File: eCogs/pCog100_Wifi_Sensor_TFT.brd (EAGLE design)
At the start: 47.5 x 28 mm, 30 parts

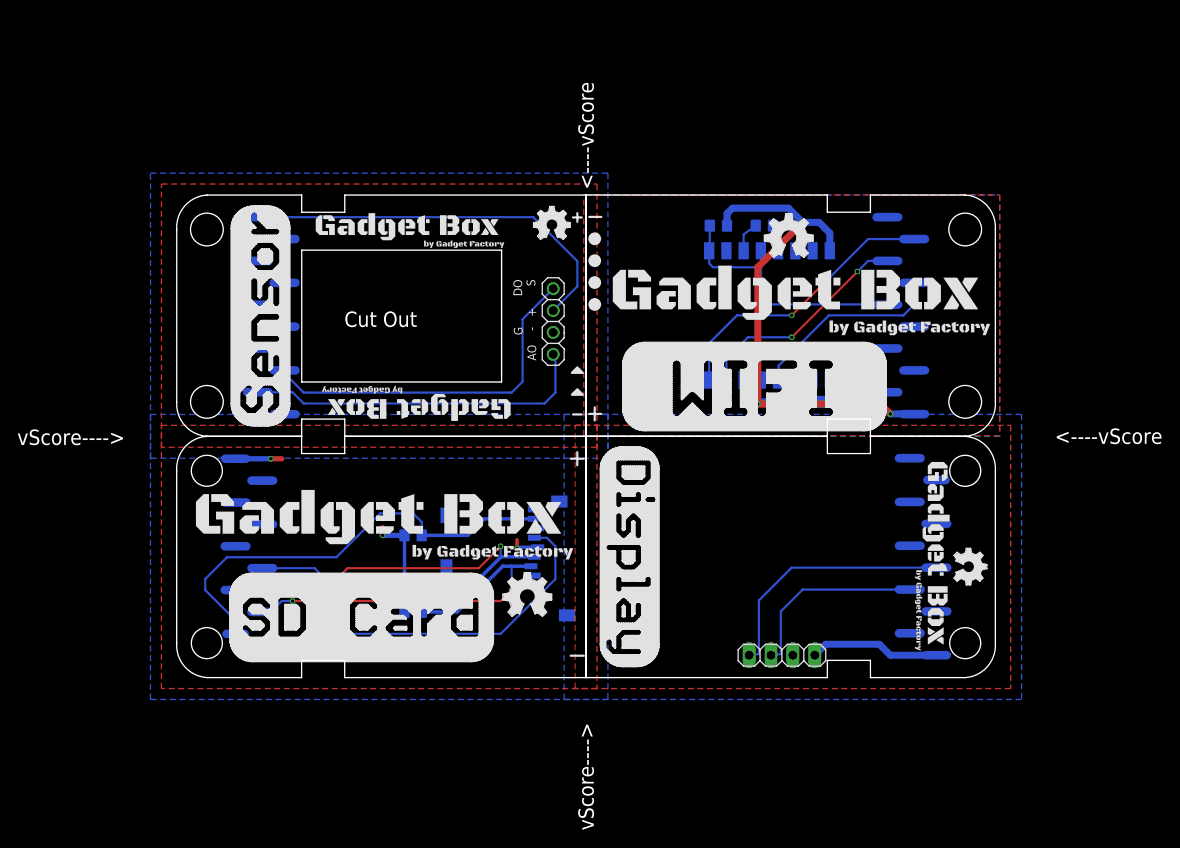
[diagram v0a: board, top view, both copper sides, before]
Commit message: pCog for Sensor Version 1.1
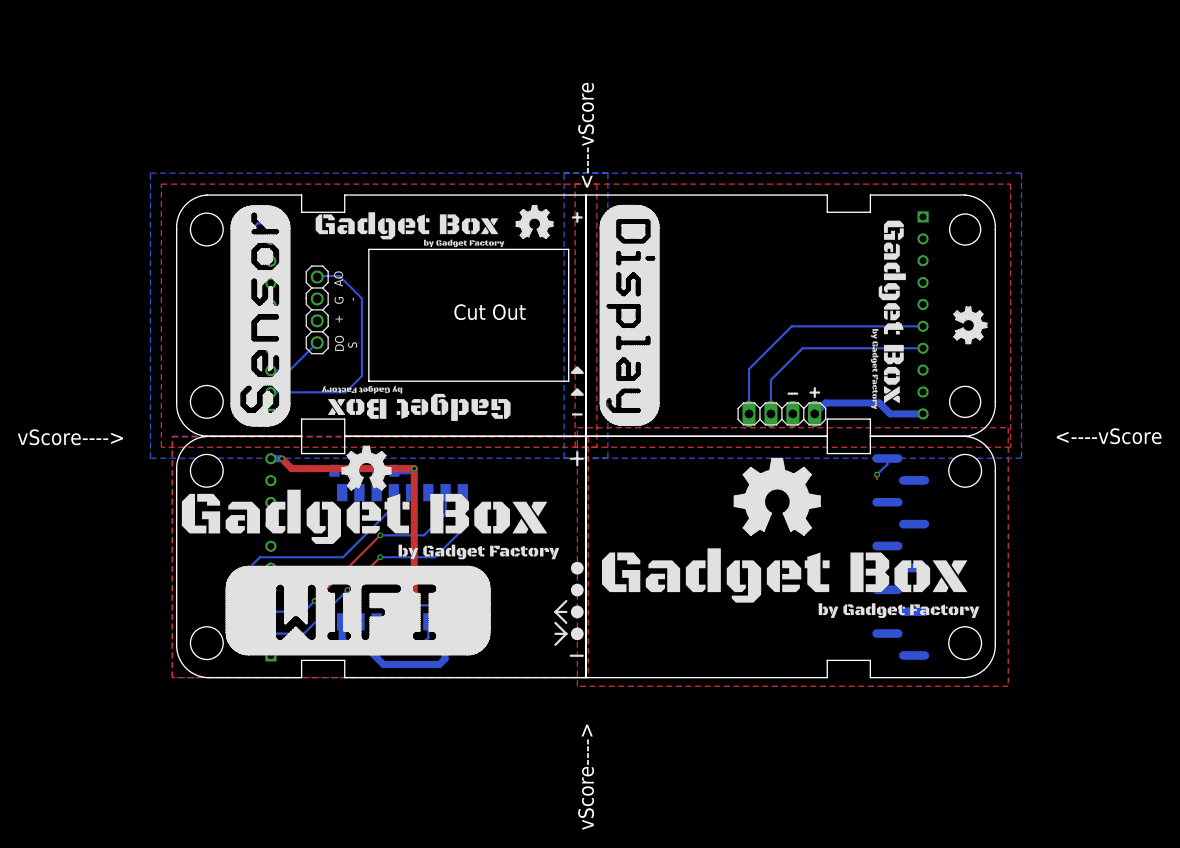
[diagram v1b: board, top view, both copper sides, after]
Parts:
- removed R5, R6, R7: 10K, GadgetFactory:0805
- removed SD1: MICROSD, adafruit:MICROSD
- ECOG: value ECOG_BUSES_ROWECOG_BUSES_SMD -> ECOG_GENERAL_ROWTHROUGHOLE; device eCogs:ECOG_BUSES_SMD -> eCogs:ECOG_GENERAL_TH
- ECOG1: value ECOG_BUSES_ROWECOG_BUSES_SMD -> ECOG_GENERAL_ROWSURFACEMOUNT; device eCogs:ECOG_BUSES_SMD -> eCogs:ECOG_GENERAL_SMD
- ECOG2: value ECOG_GENERAL_ROWECOG_GENERAL_SMD -> ECOG_GENERAL_ROWTHROUGHOLE; device eCogs:ECOG_GENERAL_SMD -> eCogs:ECOG_GENERAL_TH
- ECOG3: value ECOG_GENERAL_ROWECOG_GENERAL_SMD -> ECOG_BUSES_ROWTHROUGHHOLE; device eCogs:ECOG_GENERAL_SMD -> eCogs:ECOG_BUSES_TH
- R1, R2, R3: value 47K -> 10K; device GadgetFactory_6.0:0805 -> GadgetFactory:0805
- U$10: device GadgetFactory:GADGETBOX_SMALL -> eCogs:LEGEND_ANALOG
- U$11: device GadgetFactory:GADGETBOX_TEXT -> eCogs:LEGEND_ANALOG
- U$12, U$14, U$15: device eCogs:LEGEND_DIO -> GadgetFactory:GADGETBOX_SMALL
- U$13: device eCogs:LEGEND_DIO -> ohw-logo:OSHW_FILLX150_NOTEXT
- U$16: device ohw-logo:OSHW_FILLX200_NOTEXT -> ohw-logo:OSHW_FILLX150_NOTEXT
- U$2: device ohw-logo:OSHW_FILLX200_NOTEXT -> eCogs:LEGEND_DIO
- U$3: device GadgetFactory:GADGETBOX_SMALL -> eCogs:LEGEND_DIO
- U$4: device ohw-logo:OSHW_FILLX150_NOTEXT -> eCogs:LEGEND_DIO
- U$5: value SENSOR -> (none); device eCogs:SENSOR-HJX4 -> eCogs:LEGEND_DIO
- U$6: device eCogs:LEGEND_ANALOG -> ohw-logo:OSHW_FILLX200_NOTEXT
- U$7: device eCogs:LEGEND_ANALOG -> GadgetFactory:GADGETBOX_TEXT
- U$8: device GadgetFactory:GADGETBOX_SMALL -> ohw-logo:OSHW_FILLX350_NOTEXT
- U$9: value (none) -> SENSOR; device ohw-logo:OSHW_FILLX150_NOTEXT -> eCogs:SENSOR-HJX4
- moved R4 52.3 mm to (27.3, 3.56)
- moved U$8 52.1 mm to (65.2, 16.5)
- moved X1 46.9 mm to (29.2, 14.0), turned to 90 degrees
- moved U$4 44.3 mm to (47.0, 7.62), turned to 0 degrees
- moved U$3 41.8 mm to (47.0, 10.2), turned to 0 degrees
- moved U$5 36.2 mm to (47.0, 5.08), turned to 0 degrees
- moved U$15 35.5 mm to (83.5, 42.4), turned to 270 degrees
- moved U$7 32.3 mm to (71.1, 11.6)
- moved U$6 30.6 mm to (19.7, 21.8)
- moved U$9 28.3 mm to (14.8, 42.7), turned to 90 degrees
- moved JP1 28.0 mm to (70.7, 30.6)
- moved U$11 27.8 mm to (47.0, 33.1)
- moved U$14 26.6 mm to (28.6, 31.4)
- moved U$12 23.5 mm to (27.3, 52.4), turned to 0 degrees
- moved U$16 22.7 mm to (90.7, 43.0), turned to 270 degrees
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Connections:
- removed net SD_!CS: ECOG.SPI-CS, R3.1, SD1.2
- removed net SD_CD: SD1.CD1
- removed net SD_MISO: ECOG.SPI-MISO, R1.1, SD1.7
- removed net SD_MOSI: ECOG.SPI-MOSI, R2.1, SD1.3
- removed net SD_SCK: ECOG.SPI-SCK, SD1.5
- net 3V3: now also U$9.+; no longer R2.2, R6.2, R7.2, SD1.4, U$5.+
- net A1: now also U$9.AO; no longer U$5.AO
- net A2: now also U$9.DO/S; no longer U$5.DO/S
- net GND: now also R2.1, U$9.GND; no longer R5.1, SD1.6, SD1.MT1, SD1.MT2, U$5.GND
- net GPIO0/BOOTLOAD: now also ECOG.G2; no longer ECOG3.G2
- net N$1: now also ECOG3.I2C-SCL; no longer ECOG1.I2C-SCL
- net N$2: now also ECOG3.I2C-SDA; no longer ECOG1.I2C-SDA
- net N$3: now also R1.1; no longer R4.1
- net N$4: now also R2.2; no longer R5.2
- net N$5: now also R4.1; no longer R7.1
- net RESET: now also ECOG.G3, R3.1; no longer ECOG3.G3, R6.1
- net RX/MOSI: now also ECOG.G1; no longer ECOG3.G1
- net TX/MISO: now also ECOG.G0; no longer ECOG3.G0
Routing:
- net 3V3: track 147.2 -> 80.5 mm, vias 6 -> 4
- net SD_MISO: track 52.3 -> 0.00 mm
- net SD_!CS: track 48.7 -> 0.00 mm, vias 2 -> 0
- net SD_SCK: track 48.5 -> 0.00 mm
- net SD_MOSI: track 46.8 -> 0.00 mm, vias 2 -> 0
- net A2: track 41.7 -> 6.73 mm
- net A1: track 40.1 -> 26.7 mm
- net GND: track 0.00 -> 2.88 mm, vias 0 -> 1
- net N$2: track 29.5 -> 27.5 mm
- net GPIO0/BOOTLOAD: track 22.9 -> 24.7 mm
- net RX/MOSI: track 25.9 -> 27.5 mm
- net RESET: track 30.9 -> 32.5 mm
- net TX/MISO: track 33.3 -> 31.8 mm
- net N$1: track 22.1 -> 23.1 mm
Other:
- board text added: "Blank"
- board text added: "ecog0 v2.0"
- board text added: "ecog0.GadgetFactory.net"
- board text removed: "SPI-CS"
- board text removed: "SPI-MISO"
- board text removed: "SPI-MOSI"
- board text removed: "SPI-SCK"
- board text removed: "ecog102 v2.0"
- board text removed: "ecog102.GadgetFactory.net"
- board text removed: "uSD Card"
